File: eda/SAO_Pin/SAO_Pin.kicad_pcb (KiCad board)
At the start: 2 copper layers, 27.3 x 39.5 mm, 2 parts

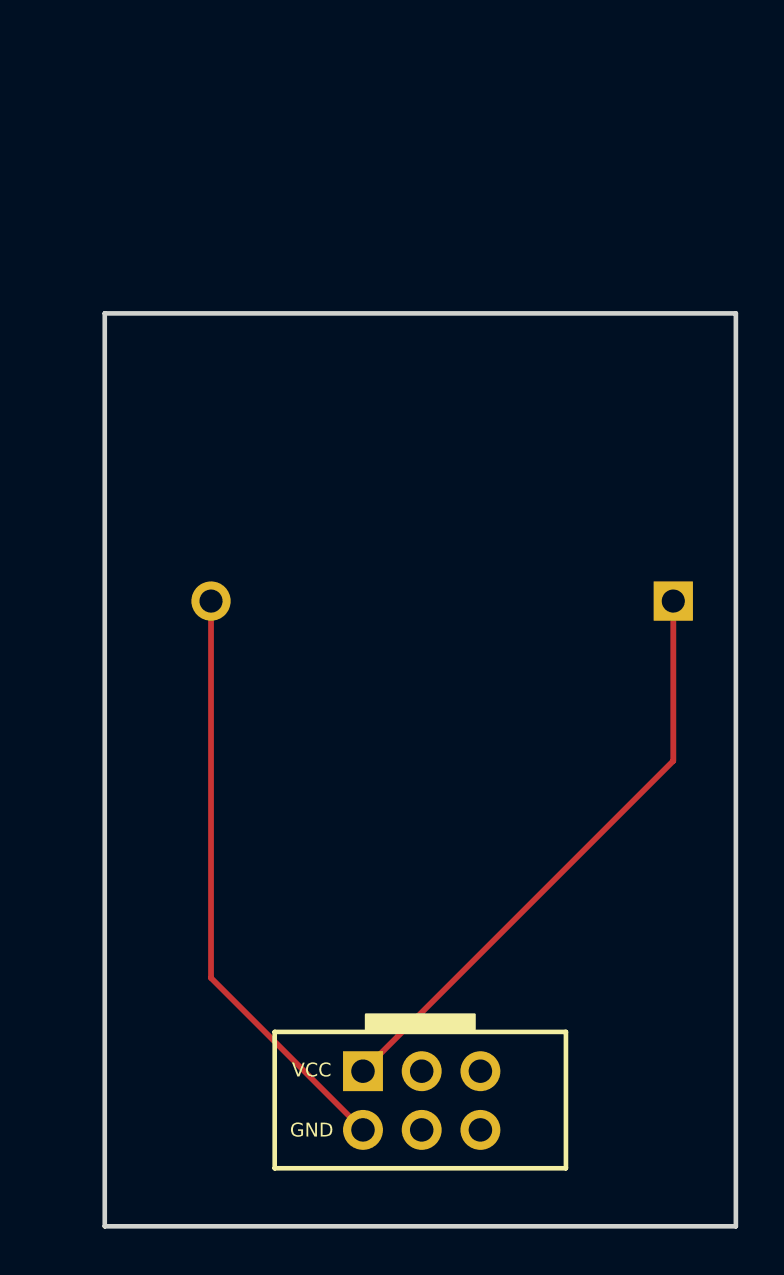
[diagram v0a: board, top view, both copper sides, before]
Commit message: pcb updates
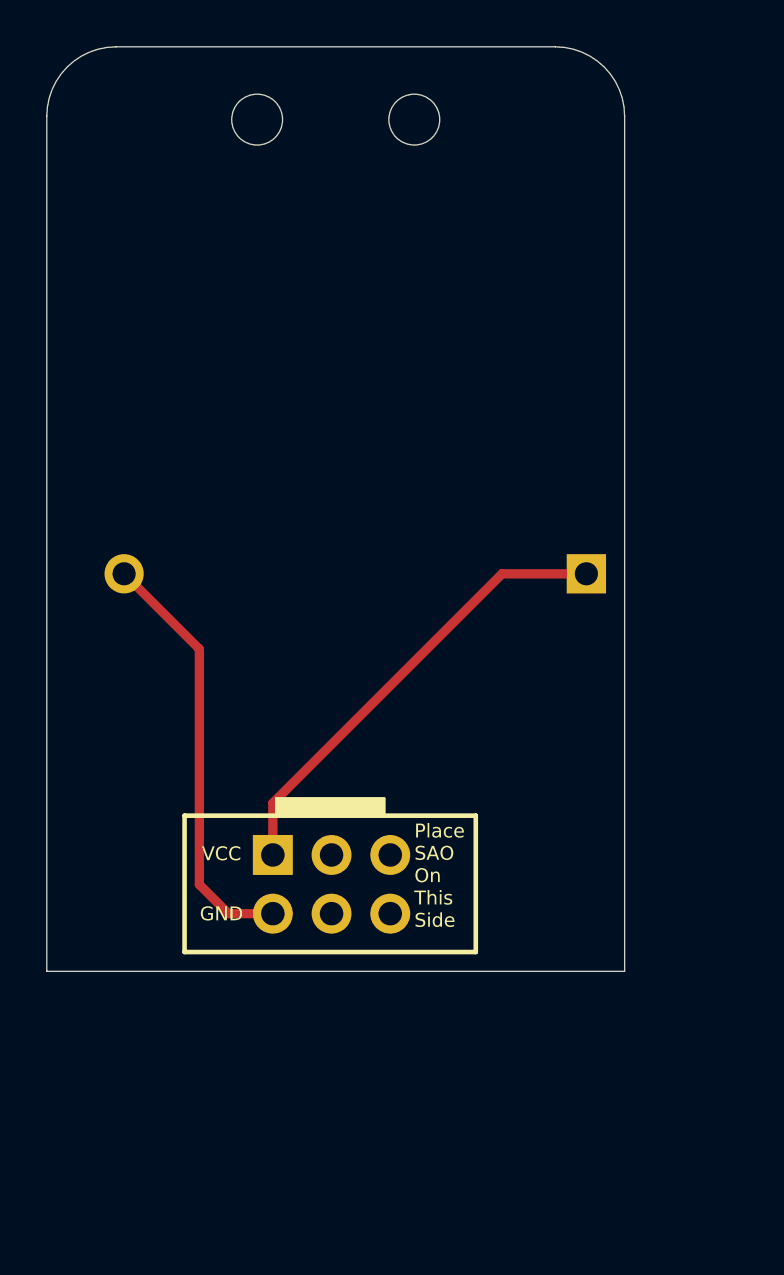
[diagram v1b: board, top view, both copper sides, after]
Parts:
- added EdgeCuts: , 0_badge:SAO_Pin_EdgeCuts, F.Cu at (139.7, 88.0)
- added G***: LOGO, 0_alt_bier:logo-alt_bier-1900dpi-5x12mm-back, F.Cu at (149.5, 81.4)
- added REF**: Broach_Clip_2cm_M2, 0_local:Broach_Clip_2cm_M2, F.Cu at (139.7, 73.2)
- BT1: footprint 0_local:BatteryHolder_CR2032-BS-2-1_Front_backsilk -> 0_local:BatteryHolder_CR2032-BS-2-1_Back_backsilk
- moved JSAO1 10.1 mm to (139.5, 106.2)
- moved BT1 3.94 mm to (127.5, 92.8)
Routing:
- net GND: track 25.6 -> 18.5 mm
- net Net-(BT1-+): track 25.9 -> 19.9 mm
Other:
- board size 27.3 x 39.5 mm -> 25 x 40 mm
- board text added: "25mm wide x 40mm tall"
- board text added: "Place 20mm Broach Pin Clasp On This Side"
- board text added: "Place Battery Connector On This Side"
- board text added: "Place SAO On This Side"
